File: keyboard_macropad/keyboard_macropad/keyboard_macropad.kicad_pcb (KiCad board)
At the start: 2 copper layers, 88 x 131 mm, 42 parts, among them J1 Conn_01x04_Pin, J2 Conn_01x04_Pin, J3 Conn_01x04_Pin, J4 Conn_01x04_Pin, SW1 SW_Push, SW10 SW_Push, SW11 SW_Push, SW12 SW_Push, SW13 SW_Push, SW14 SW_Push, SW15 SW_Push, SW16 SW_Push, SW2 SW_Push, SW3 SW_Push, SW4 SW_Push, SW5 SW_Push, SW6 SW_Push, SW7 SW_Push, SW8 SW_Push, SW9 SW_Push, U1 XIAO-RP2040-DIP

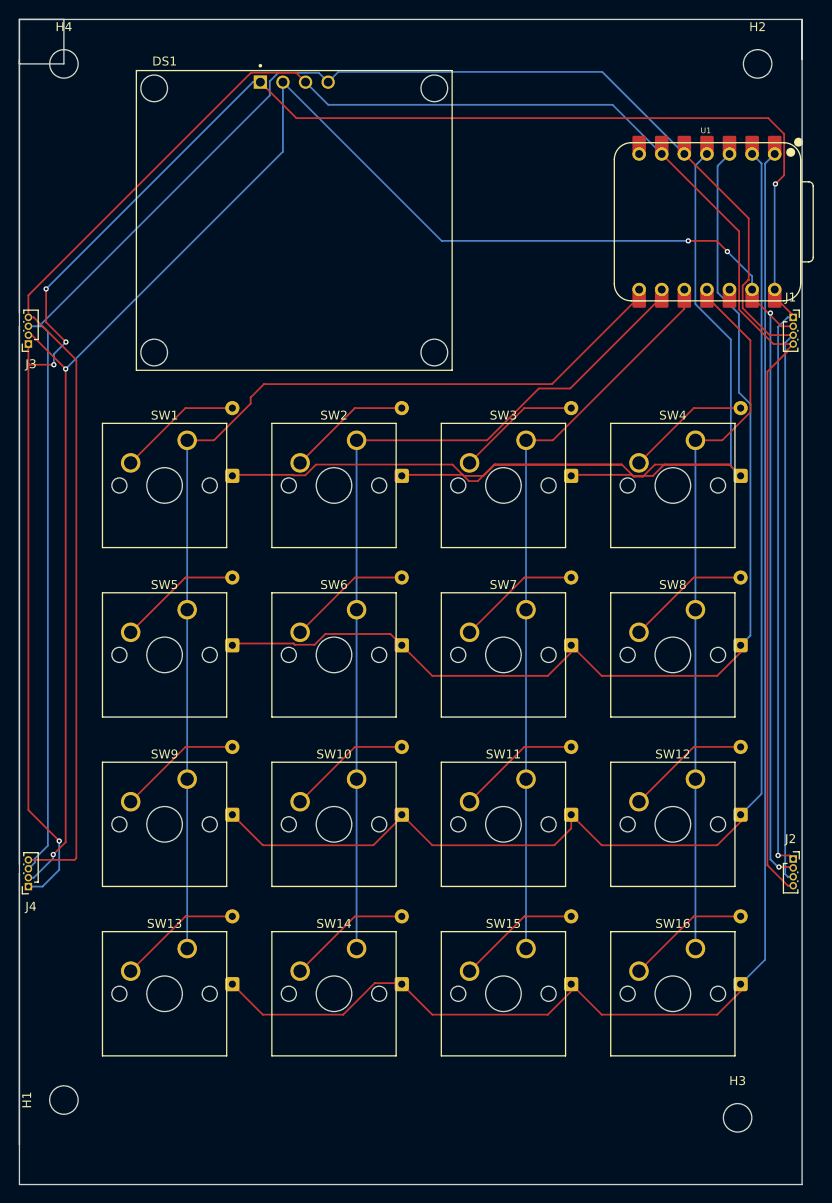
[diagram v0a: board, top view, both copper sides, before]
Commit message: updates
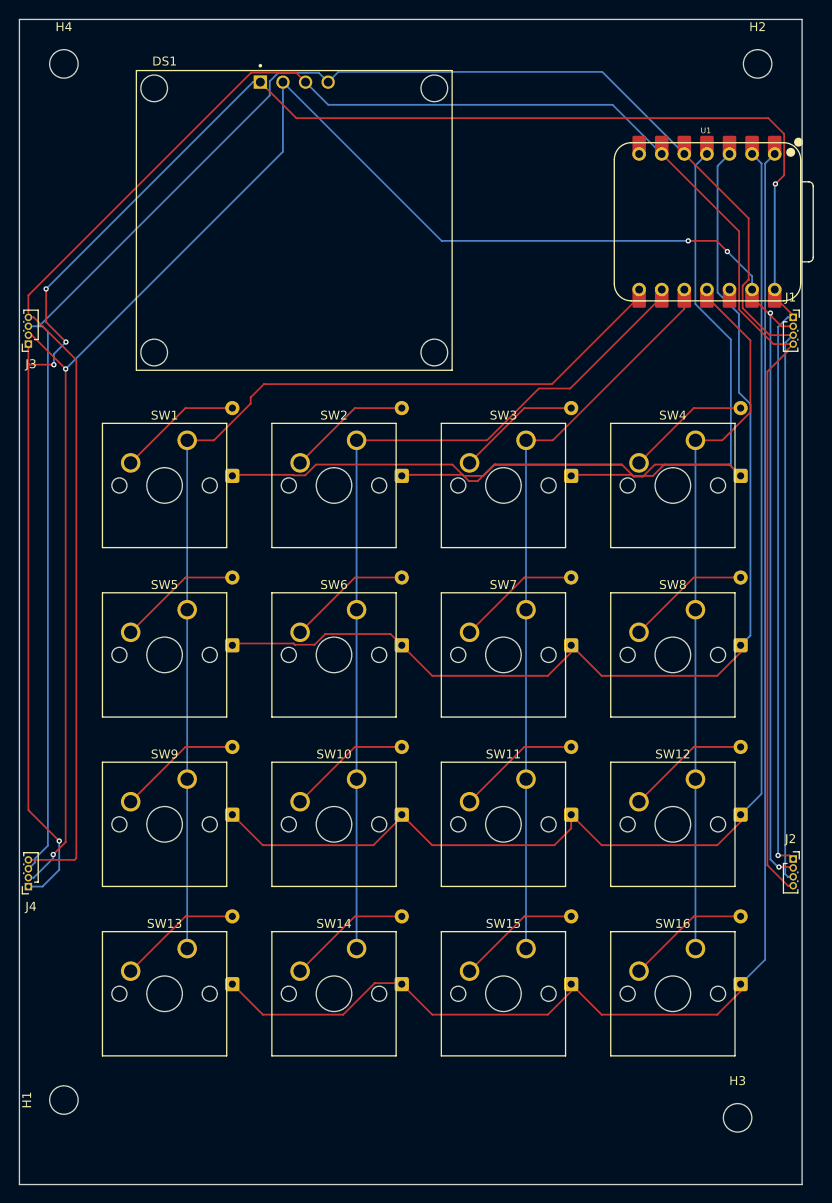
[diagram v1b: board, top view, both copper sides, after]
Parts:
- SW1, SW10, SW11, SW12, SW13, SW14, SW15, SW16, SW2, SW3, SW4, SW5, SW6, SW7, SW8, SW9: footprint Button_Switch_Keyboard:SW_Cherry_MX_1.00u_PCB -> dakshmessesaround:jiggupiggu
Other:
- outline, holes or cut-outs redrawn
